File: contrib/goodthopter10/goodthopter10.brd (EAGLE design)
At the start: 72.7 x 31.8 mm, 24 parts, among them IC1 F22X4---DA38, IC2 FT232RL-BASICSSOP, Q2 20MHz

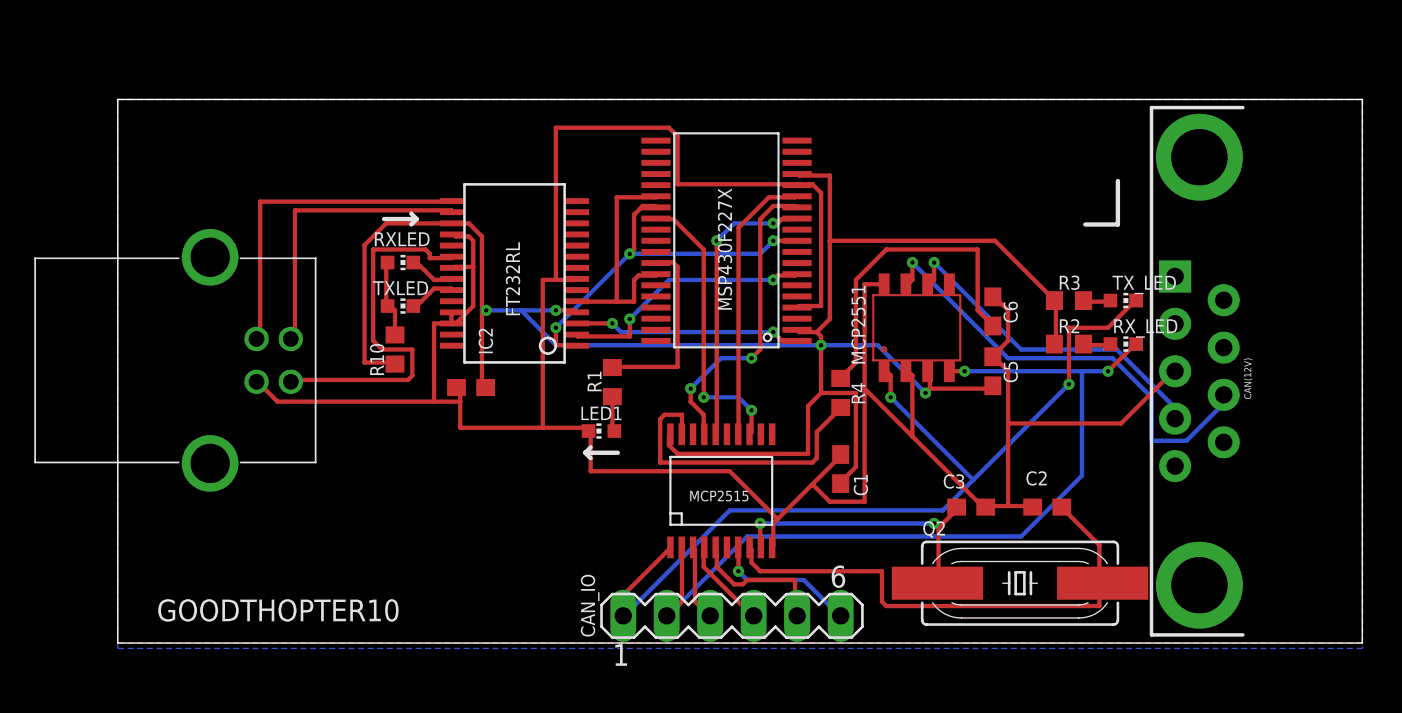
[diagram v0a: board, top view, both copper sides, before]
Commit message: Updated Routing/SCH and Produced Gerbers
git-svn-id: https://svn.code.sf.net/p/goodfet/code@1216 12e2690d-a6be-4b82-a7b7-67c4a43b65c8
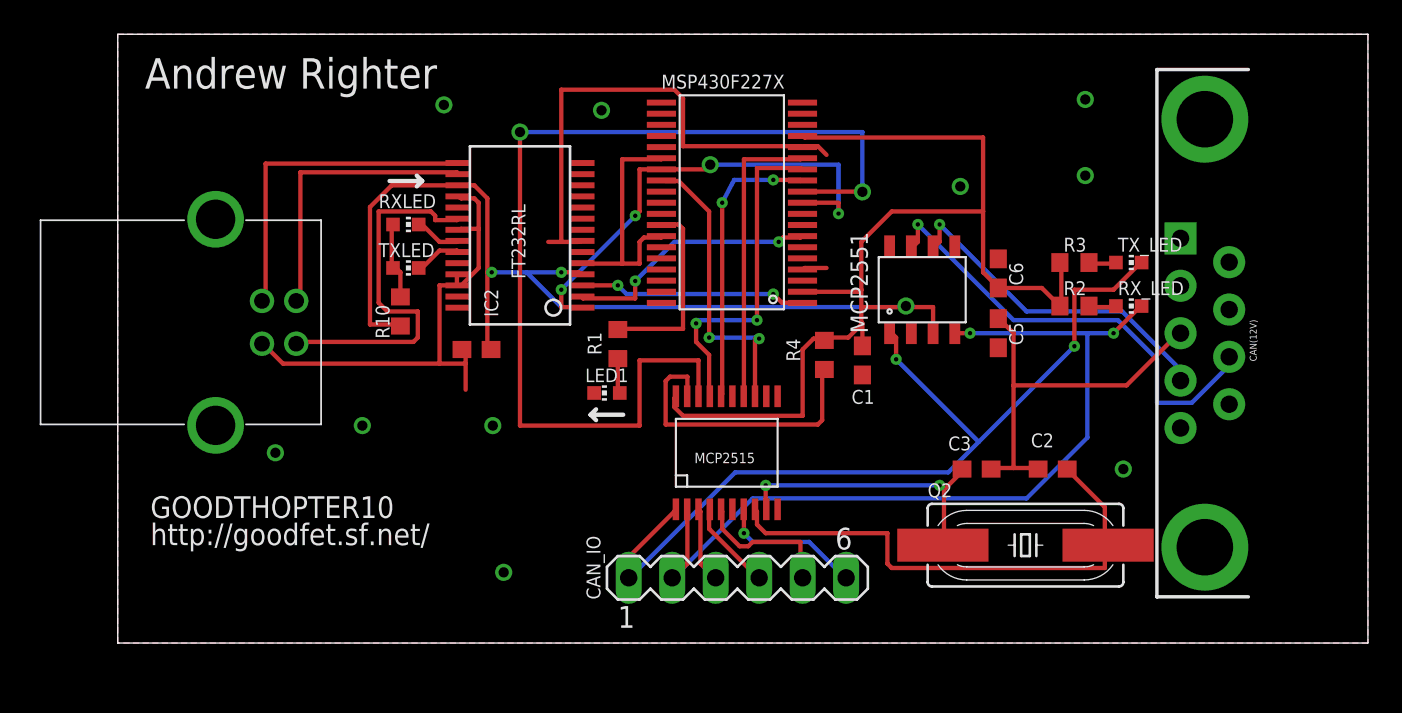
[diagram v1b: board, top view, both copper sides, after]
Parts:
- R2, R3: value 470 -> 330
- moved C1 6.48 mm to (43.5, 16.5), turned to 90 degrees
- moved R4 2.42 mm to (41.3, 16.8)
- moved 292304-2 2.25 mm to (5.71, 18.7)
- moved C2 2.25 mm to (54.6, 10.2)
- moved C3 2.25 mm to (50.2, 10.2)
- moved C5 2.25 mm to (51.4, 18.1)
- moved C6 2.25 mm to (51.4, 21.6)
- moved CAN(12V) 2.25 mm to (63.5, 18.1)
- moved CAN_IO 2.25 mm to (36.2, 3.81)
- moved IC2 2.25 mm to (23.5, 23.8)
- moved R10 2.25 mm to (16.5, 19.4)
- moved R2 2.25 mm to (55.9, 19.7)
- moved R3 2.25 mm to (55.9, 22.2)
- moved RX_LED 2.25 mm to (59.1, 19.7)
- moved TX_LED 2.25 mm to (59.1, 22.2)
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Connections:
- net N$3 renamed USBDP
- net N$4 renamed USBDM
- removed net N$11: C6.2, R4.1
- new net !CS: IC1.11, U$1.18
- net VCC: now also C6.2, R4.1
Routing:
- net GND: track 163.2 -> 83.5 mm, vias 0 -> 10
- net !CS: track 0.00 -> 60.5 mm, vias 0 -> 2
- net N$11: track 18.8 -> 0.00 mm
- net RXD: track 22.4 -> 28.7 mm, vias 3 -> 4
- net VCC: track 115.8 -> 120.6 mm, vias 4 -> 3
- net MISO: track 18.1 -> 19.9 mm
- net SCK: track 16.2 -> 17.3 mm
- net !INT: track 16.7 -> 17.5 mm
- net N$5: track 17.8 -> 17.3 mm
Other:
- board size 72.7 x 31.8 mm -> 73 x 35.6 mm
- board text added: "Andrew Righter"
- board text added: "http://goodfet.sf.net/"
